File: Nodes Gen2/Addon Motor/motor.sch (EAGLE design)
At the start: 25 parts

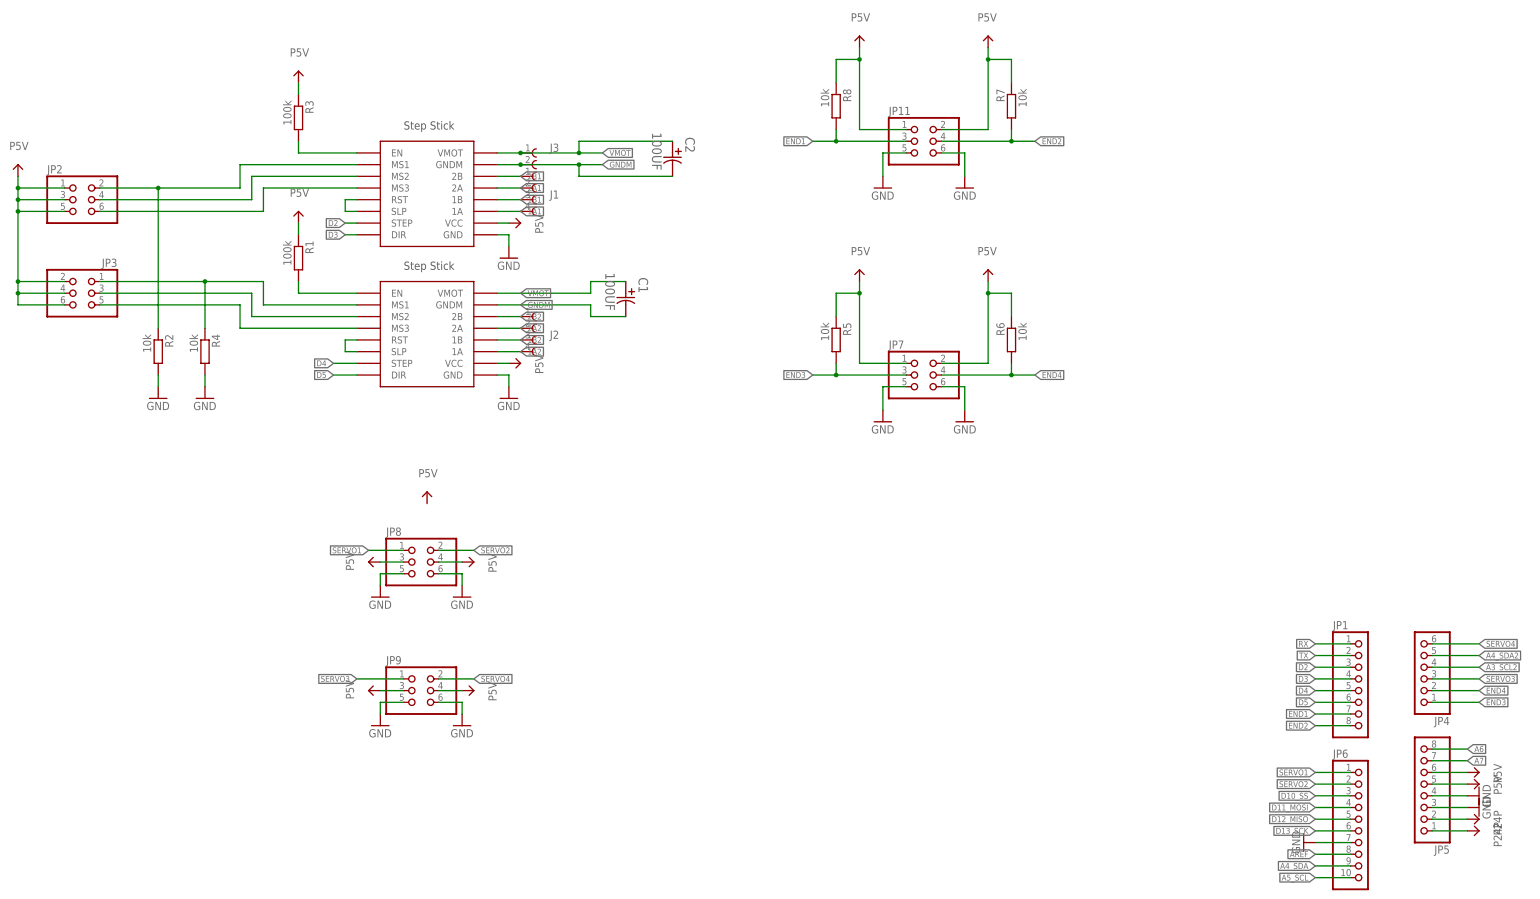
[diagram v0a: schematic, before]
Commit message: gen 2 dev + bom
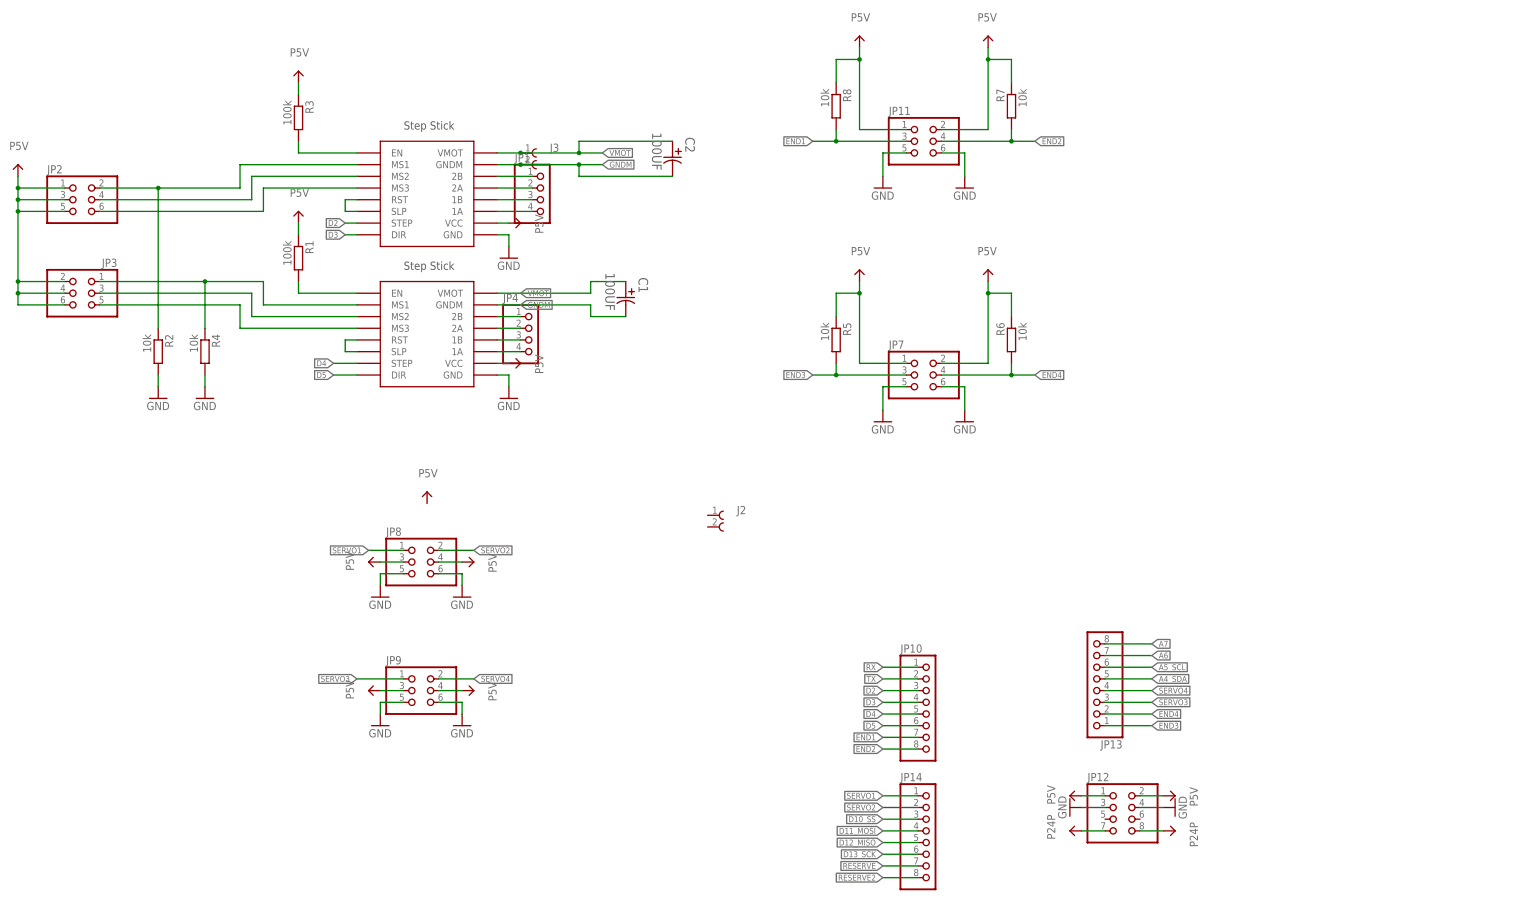
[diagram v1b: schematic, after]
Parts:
- removed J1: (no value), Eagle_TERMINAL_BLOCKS_rev16a:691312510004
- removed JP5: (no value), pinhead:PINHD-1X8
- removed JP6: (no value), pinhead:PINHD-1X10
- added JP10, JP13, JP14: (no value), pinhead:PINHD-1X8
- added JP12: (no value), pinhead:PINHD-2X4
- J2: device Eagle_TERMINAL_BLOCKS_rev16a:691312510004 -> Eagle_TERMINAL_BLOCKS_rev16a:691322310002
- JP1: device pinhead:PINHD-1X8 -> pinhead:PINHD-1X4/90
- JP4: device pinhead:PINHD-1X6 -> pinhead:PINHD-1X4/90
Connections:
- removed net 1A1: J1.4, U$2.1A
- removed net 1A2: J2.4, U$1.1A
- removed net 1B1: J1.3, U$2.1B
- removed net 1B2: J2.3, U$1.1B
- removed net 2A1: J1.2, U$2.2A
- removed net 2A2: J2.2, U$1.2A
- removed net 2B1: J1.1, U$2.2B
- removed net 2B2: J2.1, U$1.2B
- removed net A3_SCL2: JP4.4
- removed net A4_SDA2: JP4.5
- removed net A6: JP5.8
- removed net A7: JP5.7
- removed net AREF: JP6.8
- new net N$11: JP1.4, U$2.1A
- new net N$12: JP1.3, U$2.1B
- new net N$13: JP1.2, U$2.2A
- new net N$14: JP1.1, U$2.2B
- new net N$15: JP4.1, U$1.2B
- new net N$16: JP4.2, U$1.2A
- new net N$17: JP4.3, U$1.1B
- new net N$18: JP4.4, U$1.1A
- new net RESERVE: JP14.7
- new net RESERVE2: JP14.8
- net A4_SDA: now also JP13.5; no longer JP6.9
- net A5_SCL: now also JP13.6; no longer JP6.10
- net D10_SS: now also JP14.3; no longer JP6.3
- net D11_MOSI: now also JP14.4; no longer JP6.4
- net D12_MISO: now also JP14.5; no longer JP6.5
- net D13_SCK: now also JP14.6; no longer JP6.6
- net D2: now also JP10.3; no longer JP1.3
- net D3: now also JP10.4; no longer JP1.4
- net D4: now also JP10.5; no longer JP1.5
- net D5: now also JP10.6; no longer JP1.6
- net END1: now also JP10.7; no longer JP1.7
- net END2: now also JP10.8; no longer JP1.8
- net END3: now also JP13.1; no longer JP4.1
- net END4: now also JP13.2; no longer JP4.2
- net GND: now also JP12.3, JP12.4; no longer JP5.3, JP5.4, JP6.7
- net P24P: now also JP12.7, JP12.8; no longer JP5.1, JP5.2
- net P5V: now also JP12.1, JP12.2; no longer JP5.5, JP5.6
- net RX: now also JP10.1; no longer JP1.1
- net SERVO1: now also JP14.1; no longer JP6.1
- net SERVO2: now also JP14.2; no longer JP6.2
- net SERVO3: now also JP13.3; no longer JP4.3
- net SERVO4: now also JP13.4; no longer JP4.6
- net TX: now also JP10.2; no longer JP1.2
